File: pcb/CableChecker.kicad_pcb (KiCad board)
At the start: 2 copper layers, 30 x 100 mm, 8 parts, among them J2 NC3MAAH, J3 NC3FAAH, SW1 RotaryEncoder_Switch_MP, SW2 SW_SP3T, U1 ES8388

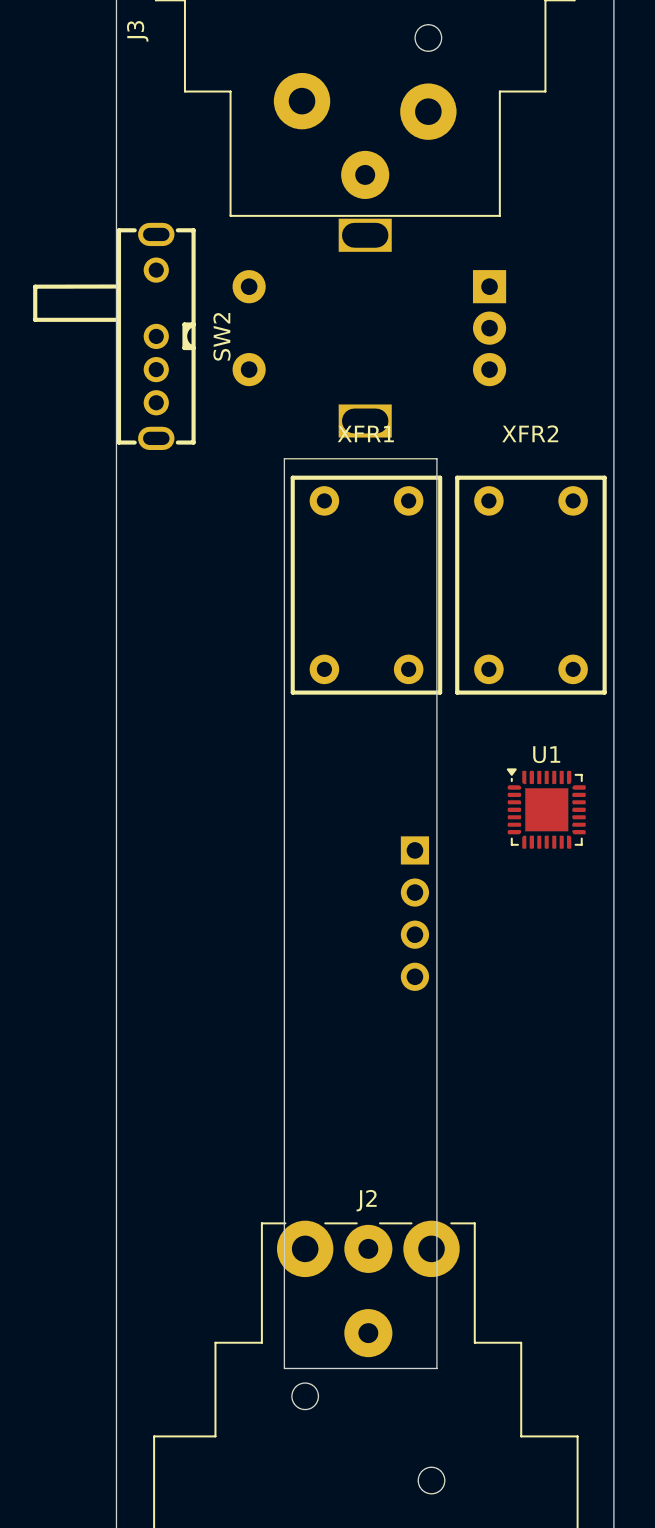
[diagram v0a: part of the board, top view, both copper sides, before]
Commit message: hardware mostly done
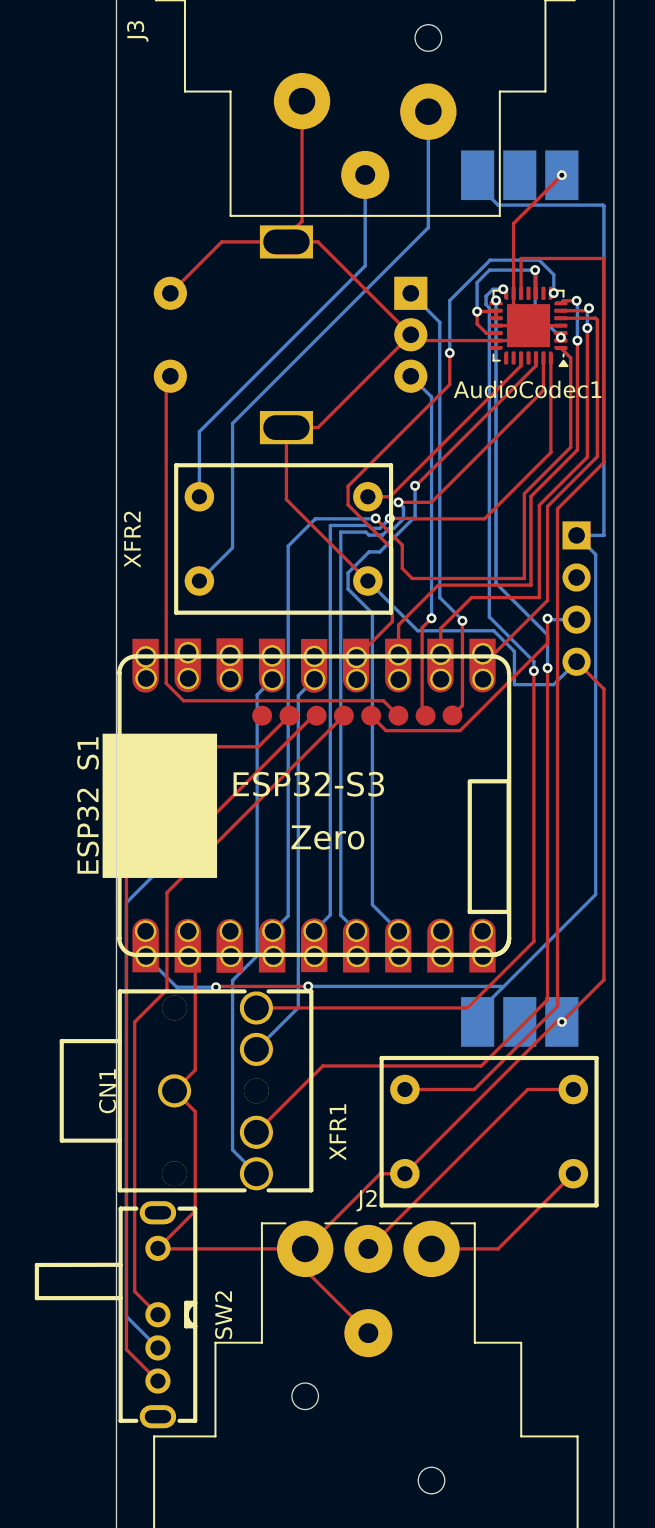
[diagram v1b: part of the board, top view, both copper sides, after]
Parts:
- added CN1: PJ-306M, easyeda2kicad:AUDIO-TH_HOOYA_PJ-306M, F.Cu at (187.0, 121.5)
- added ESP32_S1: ~, RF_Module:ESP32-S3-ZERO, F.Cu at (190.9, 104.2)
- moved SW2 59.0 mm to (183.5, 135.0)
- moved XFR1 33.8 mm to (203.5, 124.0), turned to 90 degrees
- moved AudioCodec1 29.2 mm to (205.8, 75.3), turned to 180 degrees
- moved LED1 20.6 mm to (204.9, 91.8)
- moved XFR2 15.2 mm to (191.1, 88.2), turned to 90 degrees
- moved SW1 4.77 mm to (198.8, 73.4)
- renumbered U1 to AudioCodec1
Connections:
- AudioCodec1 pad 20: Net-(U1-VMID) -> GND
- LED1 pad 1: (no net) -> +5V
- LED1 pad 3: (no net) -> GND
- LED1 pad 4: (no net) -> GND
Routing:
- net GND: track 0.00 -> 167.7 mm, vias 0 -> 2
- net +5V: track 0.00 -> 85.3 mm, vias 0 -> 2
- net LOUT1: track 0.00 -> 64.6 mm
- net Tip: track 0.00 -> 64.3 mm, vias 0 -> 2
- net Ring: track 0.00 -> 59.7 mm, vias 0 -> 2
- net MCLK: track 0.00 -> 56.2 mm, vias 0 -> 1
- net SW-3: track 0.00 -> 49.0 mm
- net CCLK: track 0.00 -> 45.9 mm, vias 0 -> 1
- net SW-2: track 0.00 -> 43.8 mm, vias 0 -> 1
- net CDATA: track 0.00 -> 43.3 mm, vias 0 -> 1
- net SW-1: track 0.00 -> 41.9 mm
- net CE: track 0.00 -> 40.9 mm, vias 0 -> 1
- net ASDOUT: track 0.00 -> 34.8 mm, vias 0 -> 2
- net Net-(J3-Pad2): track 0.00 -> 34.0 mm
- net RE-SW: track 0.00 -> 33.4 mm
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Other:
- board text added: "Joshua Wolfson"

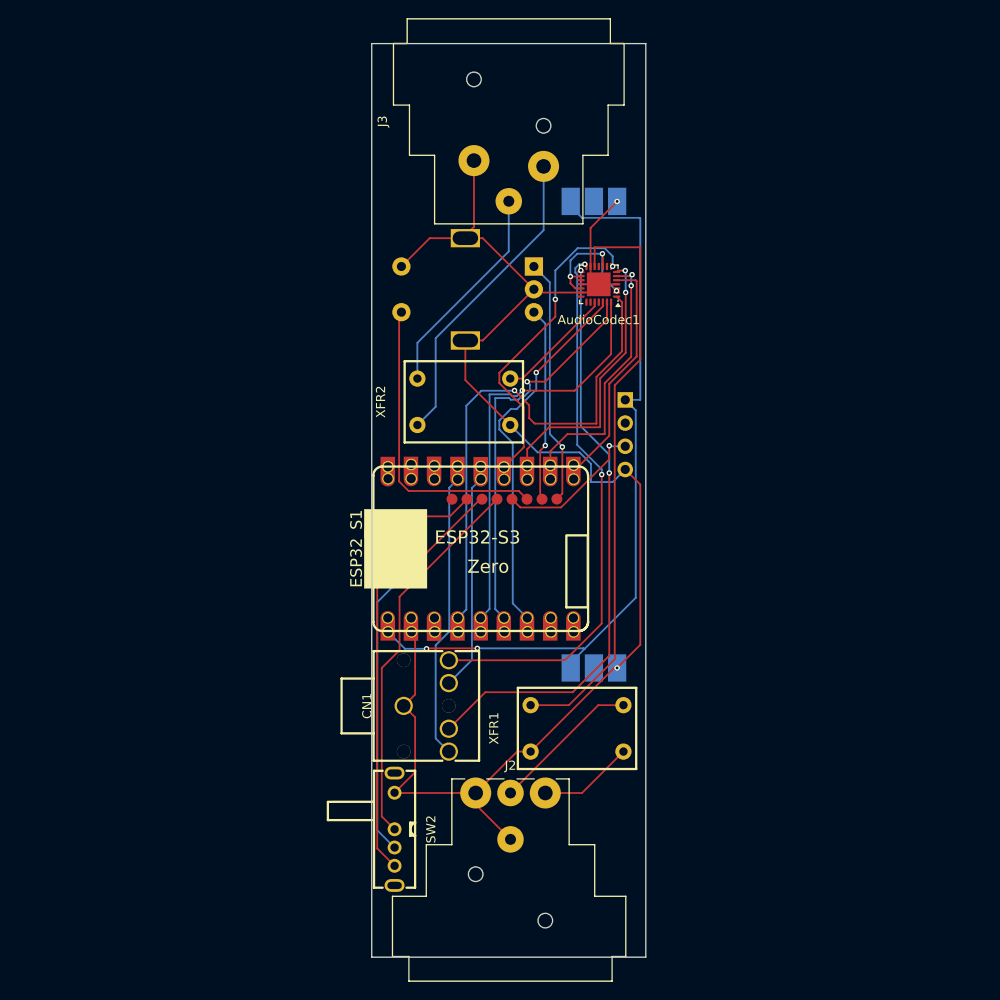
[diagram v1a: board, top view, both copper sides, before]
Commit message: finished hardware
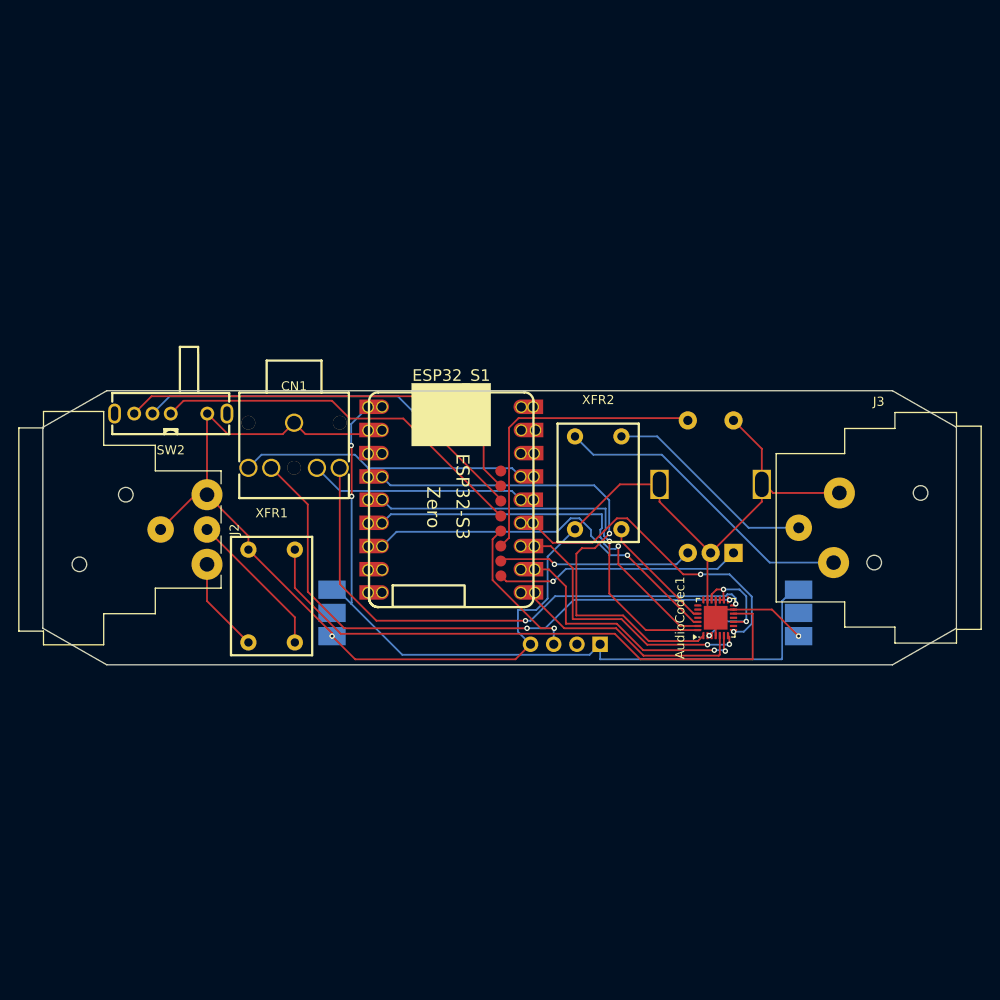
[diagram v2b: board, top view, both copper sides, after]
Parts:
- moved J3 54.1 mm to (232.2, 98.2), turned to 0 degrees
- moved SW2 51.7 mm to (159.0, 89.5), turned to 180 degrees
- moved J2 43.9 mm to (163.0, 98.4), turned to -90 degrees
- moved AudioCodec1 38.7 mm to (218.7, 111.8), turned to 90 degrees
- moved SW1 38.2 mm to (220.6, 104.8), turned to 90 degrees
- moved XFR1 36.4 mm to (170.0, 109.5), turned to 0 degrees
- moved CN1 32.0 mm to (172.5, 93.0), turned to 0 degrees
- moved LED1 19.3 mm to (202.2, 110.9), turned to 90 degrees
- moved XFR2 17.2 mm to (205.8, 97.1), turned to 0 degrees
- moved ESP32_S1 7.43 mm to (189.8, 96.9), turned to 0 degrees
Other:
- board size 30 x 100 mm -> 100 x 30 mm
